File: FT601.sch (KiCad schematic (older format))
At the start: 20 parts, among them U1 FT601, U2 ESD7016, U5 Si5351, X1 GSB443133HR, Y1 FL3000027, Y2 ABM11-141-26.000MHZ

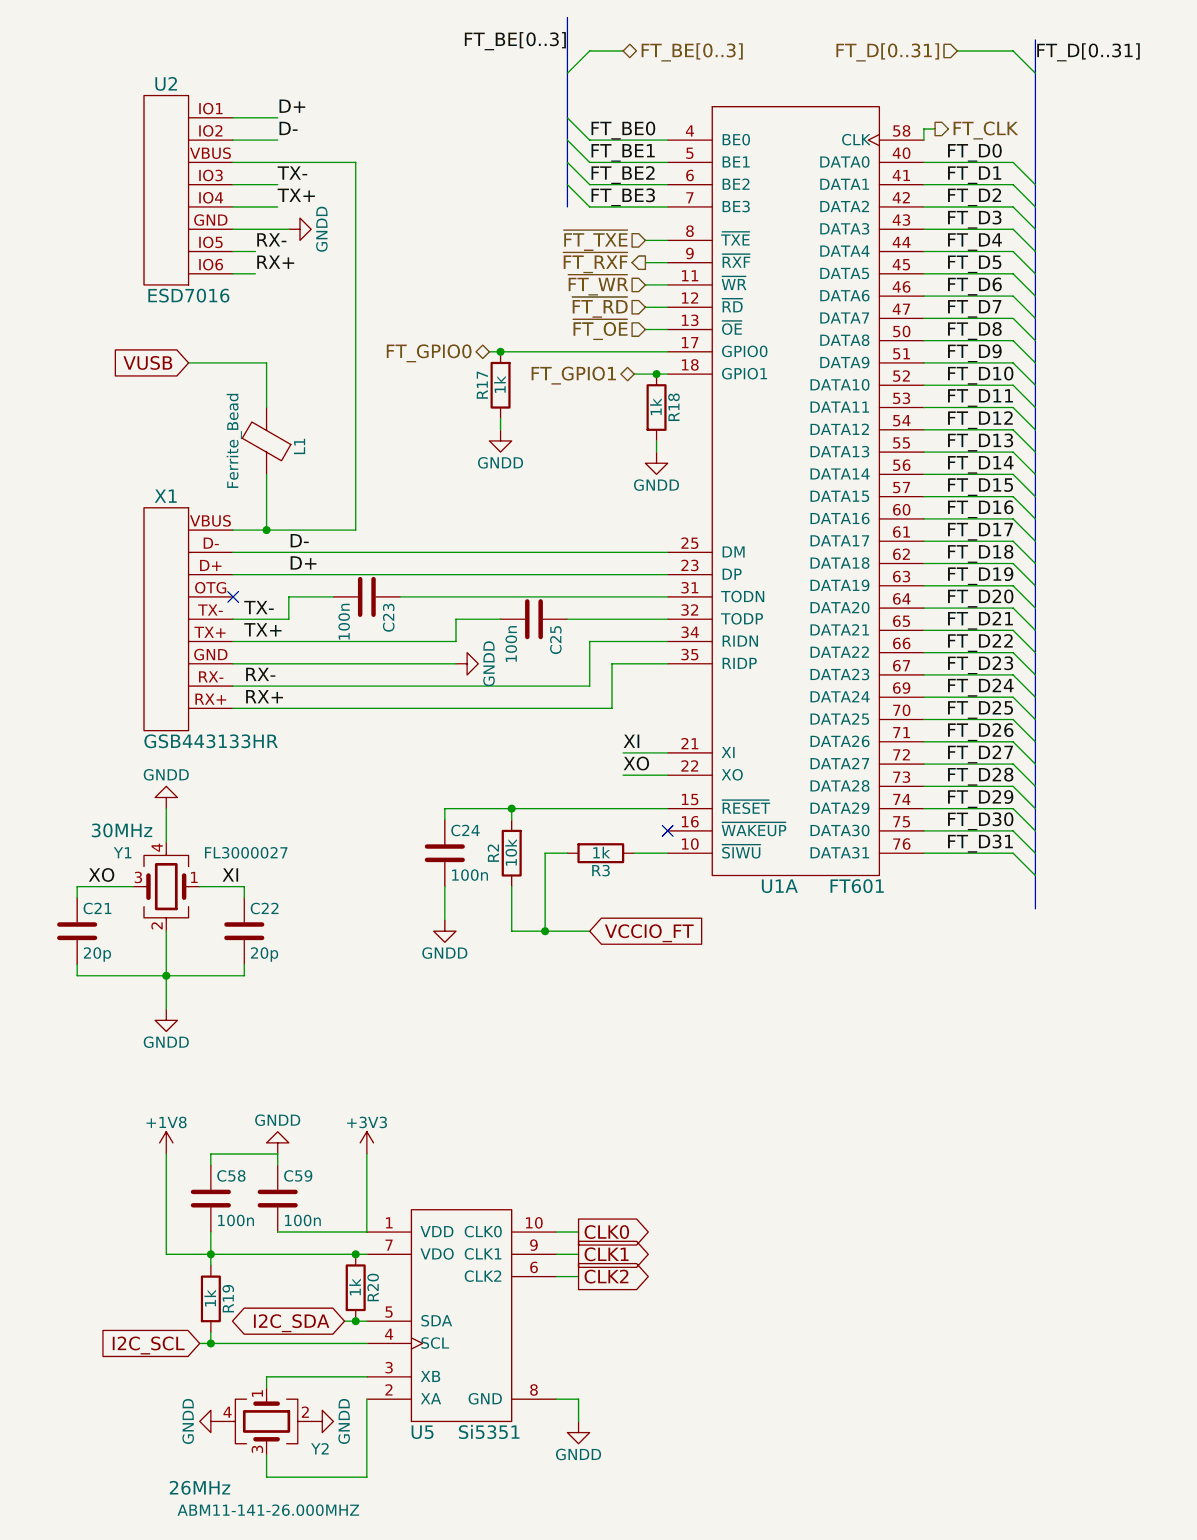
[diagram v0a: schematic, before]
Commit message: Schematic is done except RF.
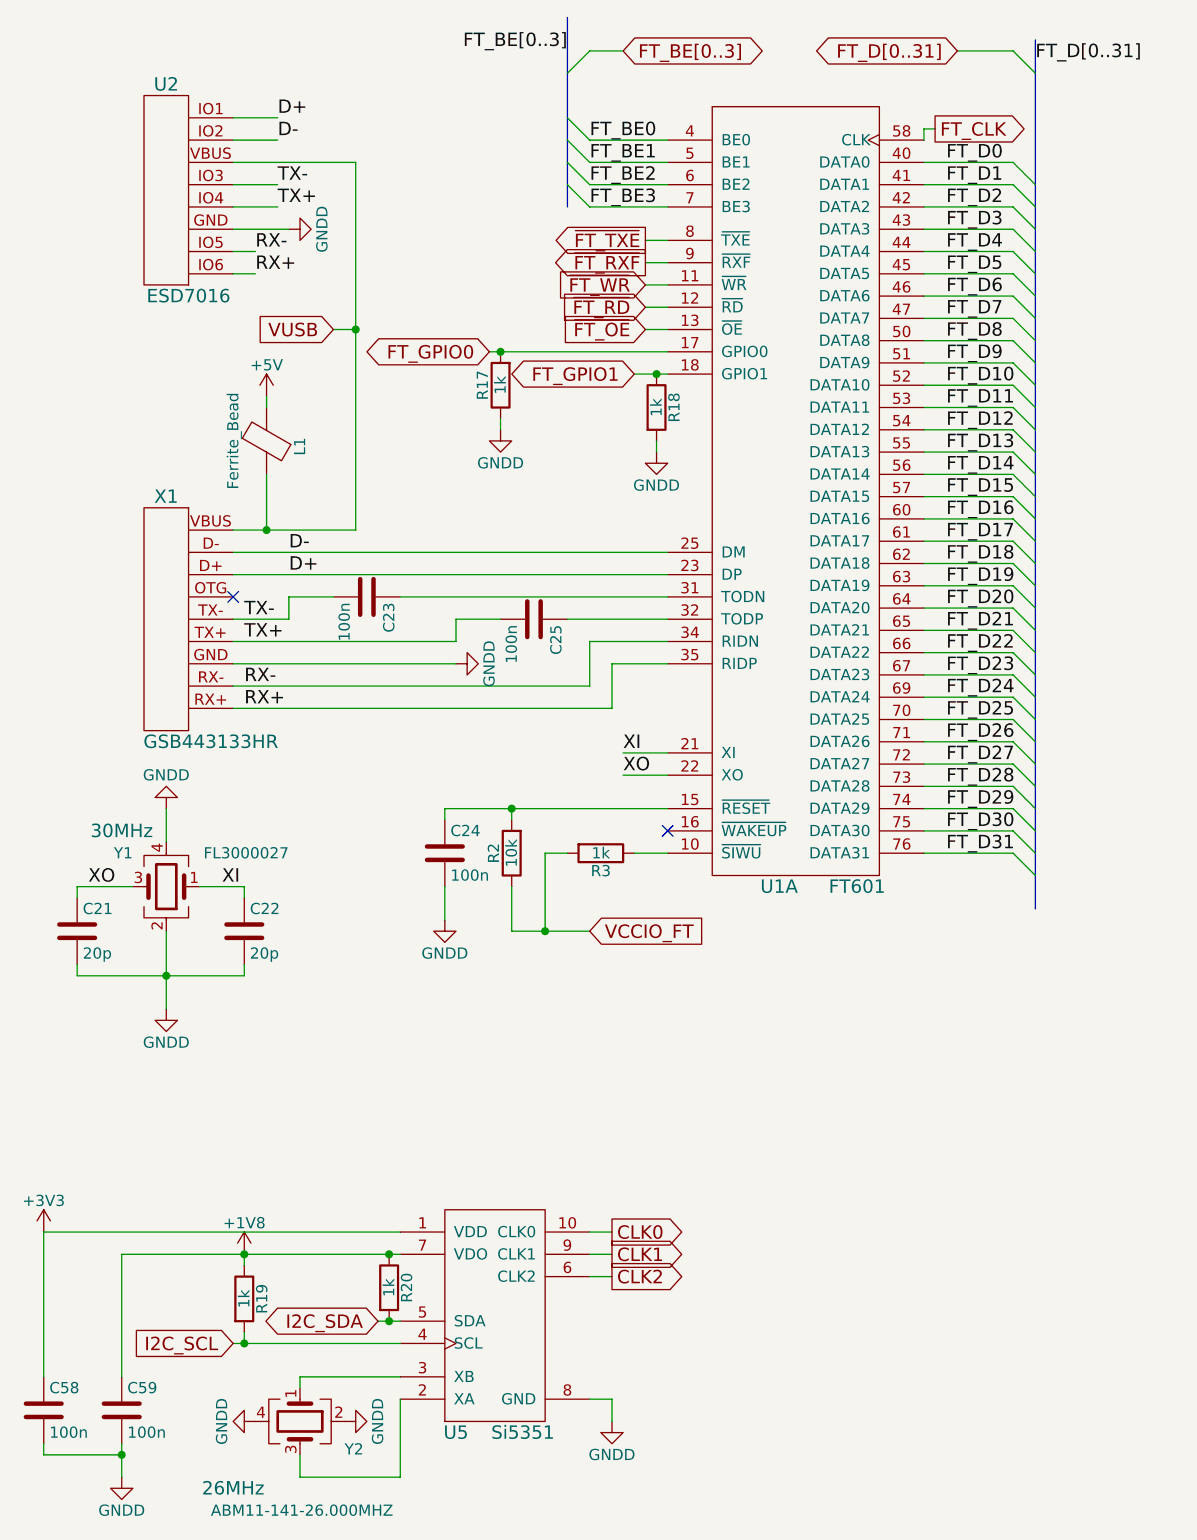
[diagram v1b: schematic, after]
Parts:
- C21, C22, C23, C24, C25, C58, C59: footprint Capacitors_SMD:C_0603_HandSoldering -> Capacitors_SMD:C_0402
- R17, R18, R19, R2, R20, R3: footprint Resistors_SMD:R_0603_HandSoldering -> Resistors_SMD:R_0402
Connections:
- net +1V8: now also C59.1; no longer C58.2
- net +3V3: now also C58.1; no longer C59.2
- net GNDD: now also C58.2, C59.2; no longer C58.1, C59.1
- net VUSB: now also L1.1, U2.VBUS, X1.VBUS; no longer L1.2
- new net +5V: L1.2
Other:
- moved on the sheet: C58, C59, R19, R20, U5, Y2
